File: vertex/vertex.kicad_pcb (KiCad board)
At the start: 2 copper layers, 34 x 29 mm, 7 parts, among them K1 CONN_3, P1 CONN_6, P2 CONN_6, P3 CONN_6, P4 CONN_1, P5 CONN_1, P6 CONN_1

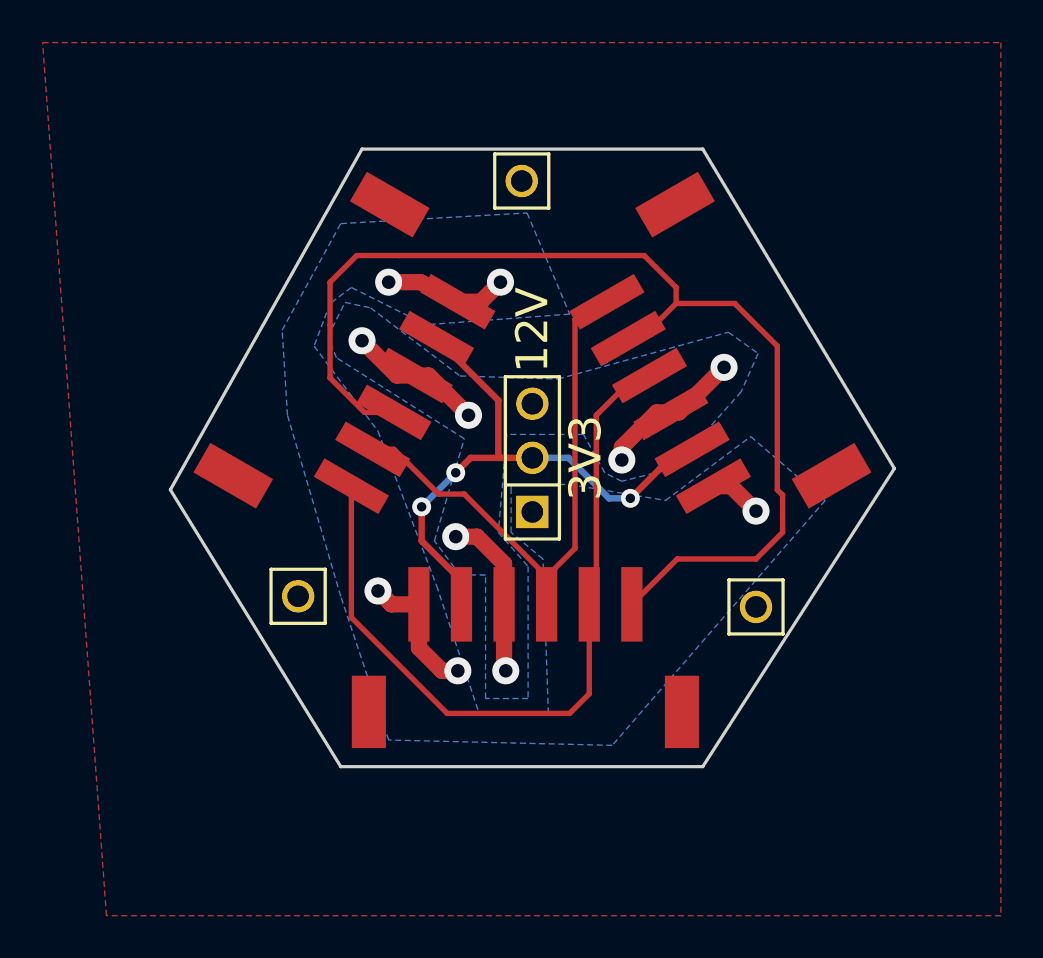
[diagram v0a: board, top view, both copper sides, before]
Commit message: Hack Manhattan Color Life boards final version
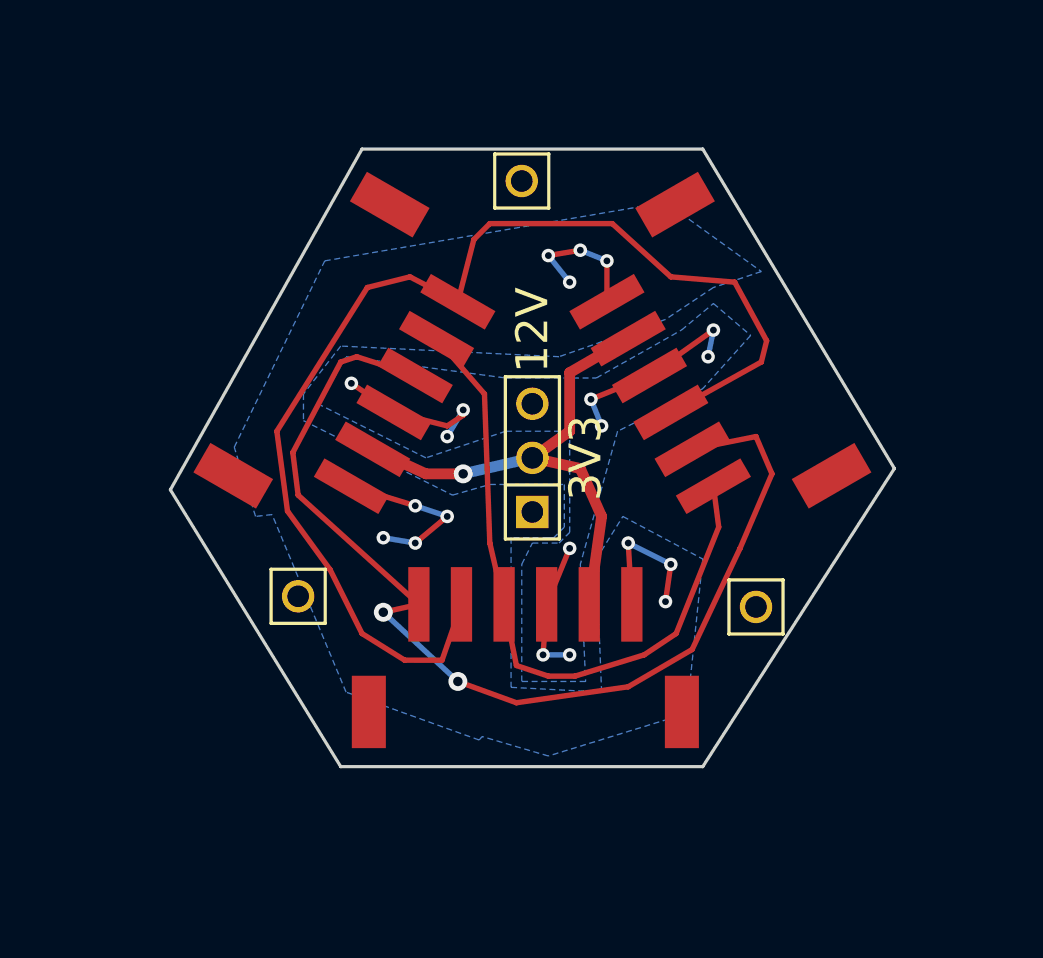
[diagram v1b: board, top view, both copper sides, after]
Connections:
- P1 pad 1: GND -> N-000009
- P1 pad 2: +3.3V -> N-000002
- P1 pad 3: +12V -> N-000003
- P1 pad 4: N-000005 (its old number) -> +12V
- P1 pad 5: N-000004 -> +3.3V
- P1 pad 6: N-000006 (its old number) -> GND
- P2 pad 1: GND -> N-000003
- P2 pad 2: +3.3V -> N-000009
- P2 pad 3: +12V -> N-000002
- P2 pad 4: N-000004 -> +12V
- P2 pad 5: N-000006 (its old number) -> +3.3V
- P2 pad 6: N-000005 (its old number) -> GND
- P3 pad 1: GND -> N-000002
- P3 pad 2: +3.3V -> N-000003
- P3 pad 3: +12V -> N-000009
- P3 pad 4: N-000006 (its old number) -> +12V
- P3 pad 5: N-000005 (its old number) -> +3.3V
- P3 pad 6: N-000004 -> GND
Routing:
- net N-000002: track 0.00 -> 55.6 mm
- net N-000006 (its old number): track 52.2 -> 0.00 mm
- net N-000009: track 0.00 -> 50.4 mm, vias 0 -> 2
- net N-000004: track 36.1 -> 0.00 mm
- net N-000003: track 0.00 -> 31.7 mm
- net N-000005 (its old number): track 27.7 -> 0.00 mm
- net GND: track 14.8 -> 21.5 mm, vias 5 -> 11
- net +3.3V: track 27.5 -> 24.9 mm, vias 3 -> 1
- net +12V: track 21.3 -> 23.3 mm, vias 6 -> 10
- removed copper zone on F.Cu, net GND
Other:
- net class lowpower: trace_width 0.3048 -> 0.508
- net class power: via_dia 1.27 -> 0.635; via_drill 0.762 -> 0.381
- rule via_min_drill: 0.508 -> 0.3048
- rule via_min_size: 0.889 -> 0.6096
